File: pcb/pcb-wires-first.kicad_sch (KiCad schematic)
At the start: 44 parts, among them J4 Conn_01x02, J5 Conn_01x02, J6 Conn_01x04, J8 I2C, SW7 set, SW8 reset, SW9 toggle, U2 SLG47115V, U3 R-78C3.3-1.0

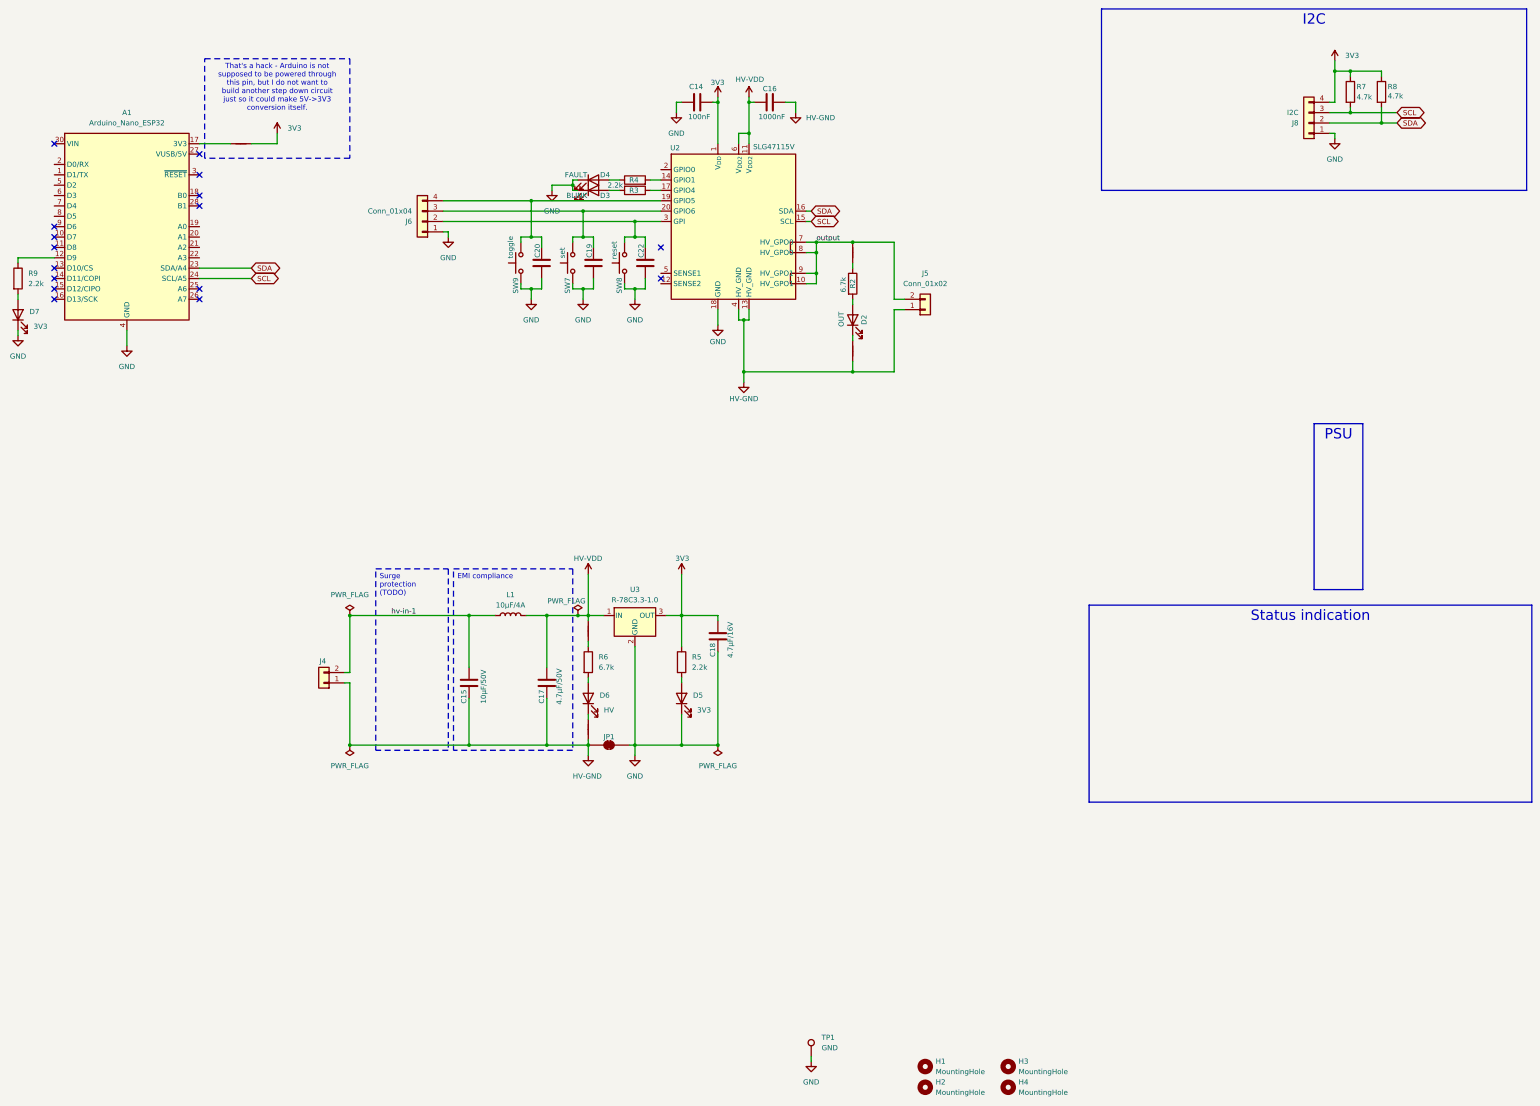
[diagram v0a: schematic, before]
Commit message: Some more cleanup.
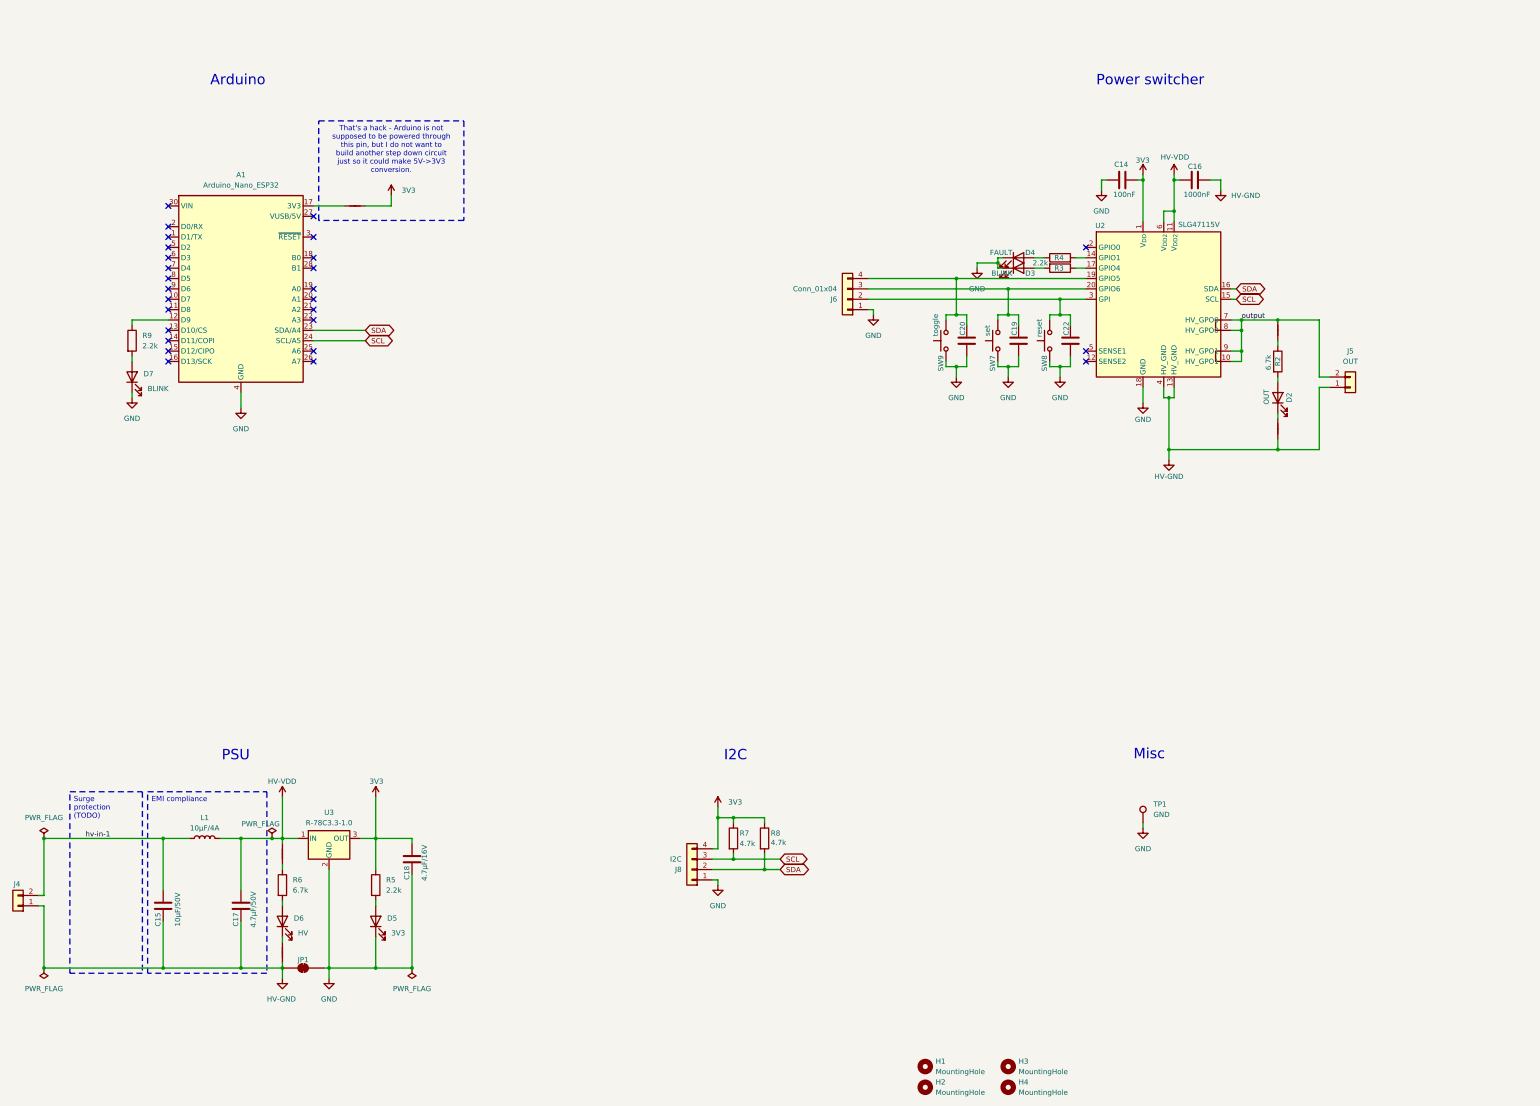
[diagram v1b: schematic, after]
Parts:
- D7: value 3V3 -> BLINK
- J5: value Conn_01x02 -> OUT
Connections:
- no-connect marks 16 -> 27
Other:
- note added: "Arduino"
- note added: "I2C"
- note added: "Misc"
- note added: "PSU"
- note added: "Power switcher"
- moved on the sheet: A1, C14, C15, C16, C17, C18, C19, C20, C22, D2, D3, D4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

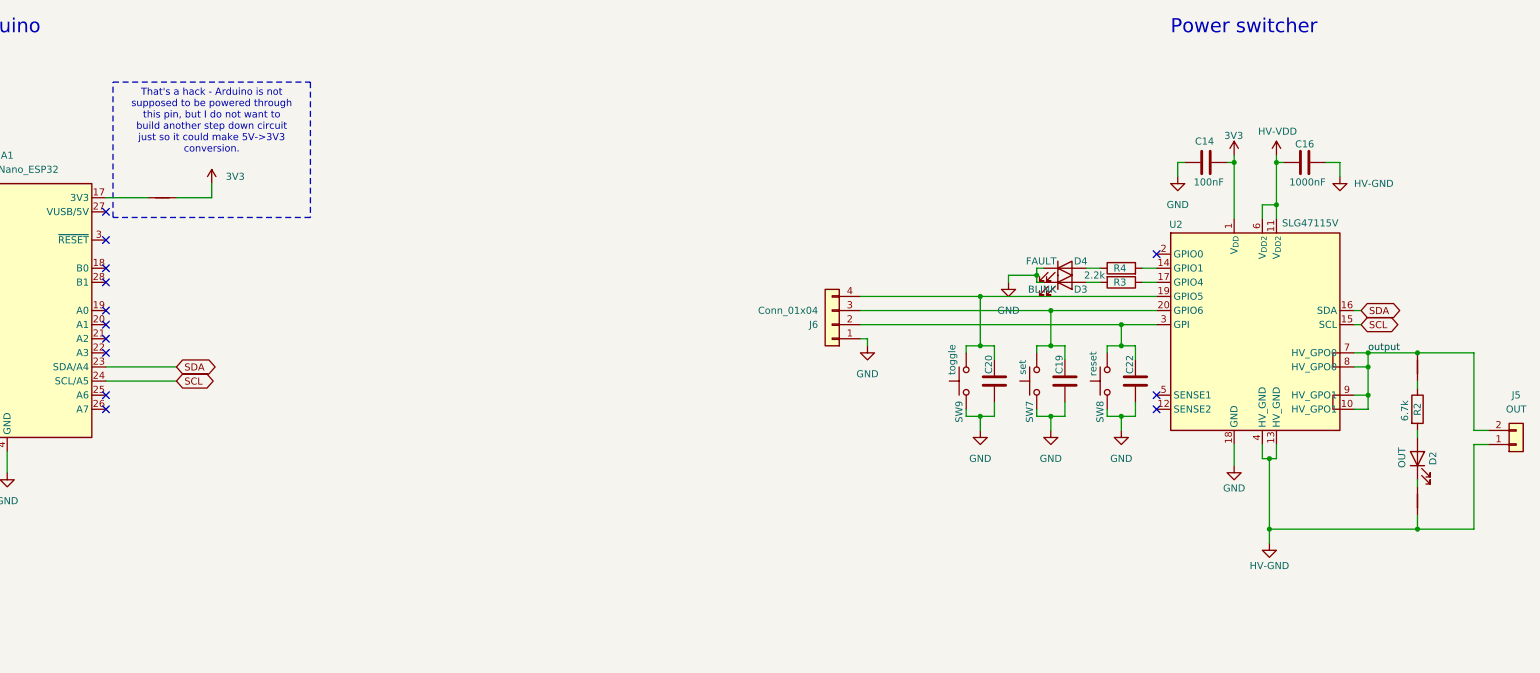
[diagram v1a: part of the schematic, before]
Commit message: Updating to new libs.
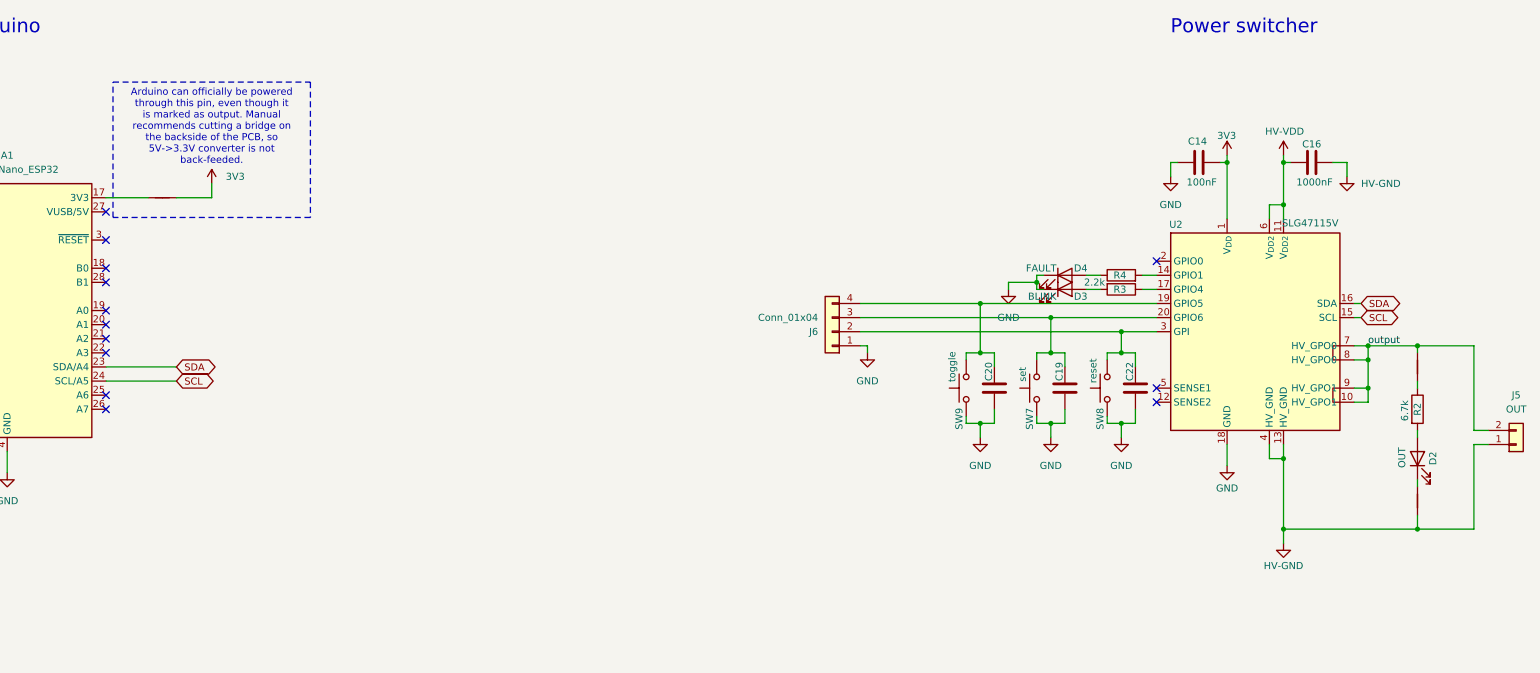
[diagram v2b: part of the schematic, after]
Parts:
- H1, H2, H3, H4: footprint Local:MountingHole_3.2mm_M3 -> MountingHole:MountingHole_3.2mm_M3_NoCopper
- U2: symbol local-lib:SLG47115V -> CPLD_Renesas:SLG47115V
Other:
- moved on the sheet: C14, C16, C19, C20, C22, D3, D4, J6, R3, R4, SW7, SW8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
